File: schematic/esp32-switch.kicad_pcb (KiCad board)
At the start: 2 copper layers, 80 x 100 mm, 27 parts, among them J1 Direction, J11 Bouton 5v, J17 Bouton Batterie, J2 + - home, J3 a b x y, J4 L R ZL ZR, J5 Joy D, J6 Joy G, J7 Moteur vibration, J8 Batterie, Q1 BC547, U1 ESP32-DevKitC

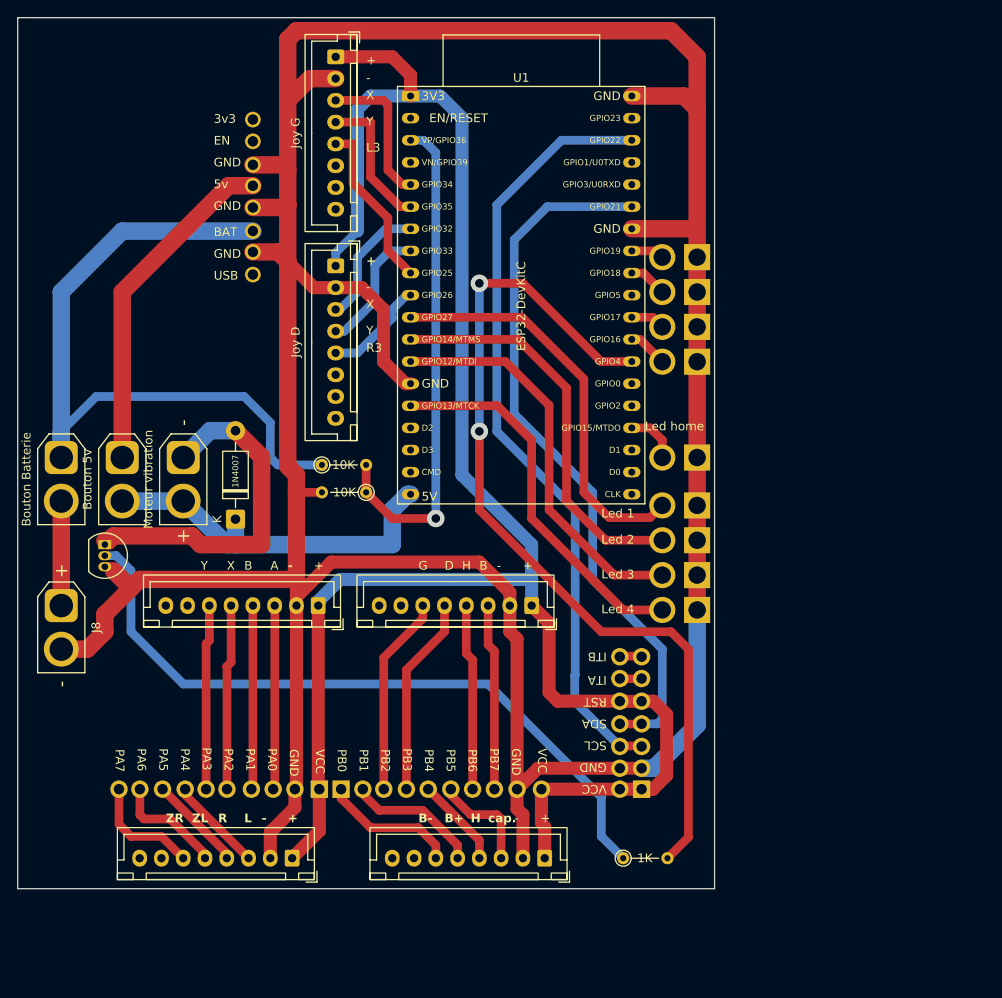
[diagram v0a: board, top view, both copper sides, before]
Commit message: changement de pcb
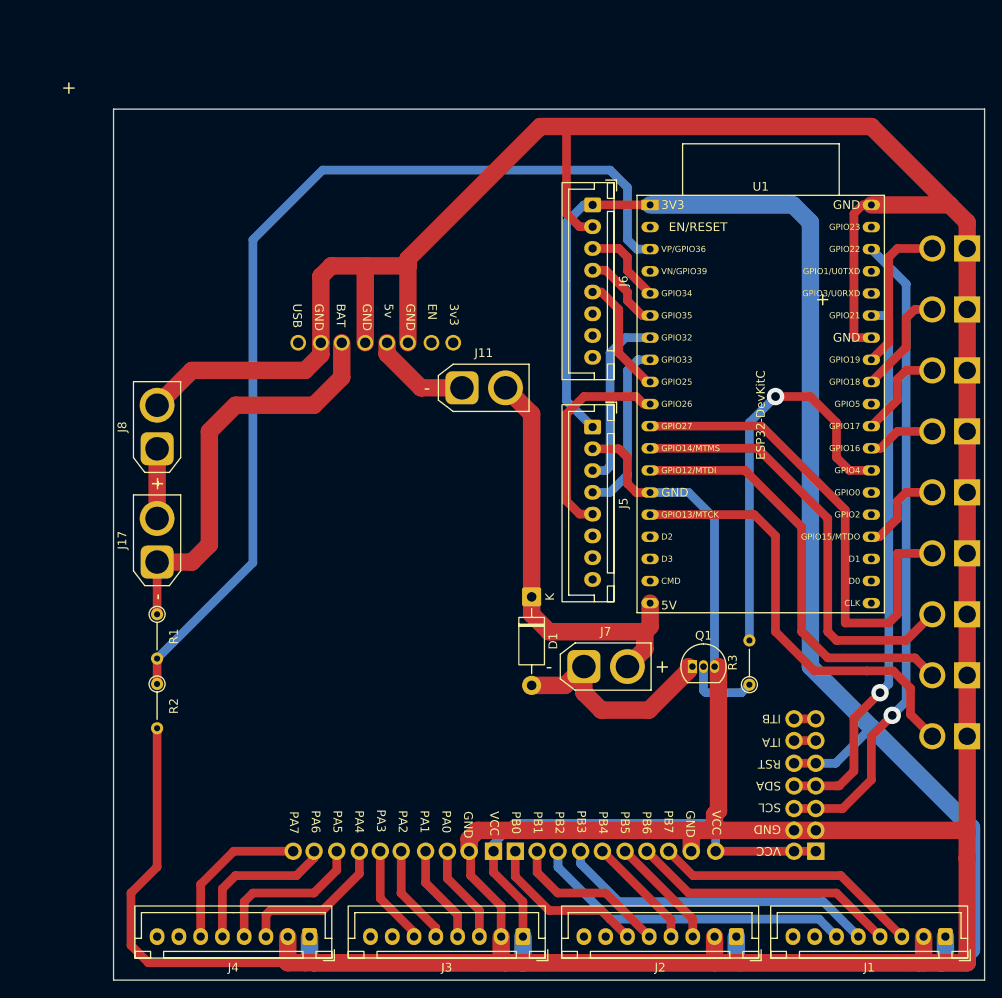
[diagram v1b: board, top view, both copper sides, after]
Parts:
- moved Q1 68.9 mm to (205.5, 105.0), turned to 0 degrees
- moved J1 60.8 mm to (234.5, 136.0)
- moved U2 57.4 mm to (187.0, 43.3), turned to -90 degrees
- moved J7 51.9 mm to (193.0, 105.0), turned to 0 degrees
- moved J3 44.7 mm to (186.0, 136.0)
- moved J11 39.8 mm to (179.0, 73.0), turned to 0 degrees
- moved D1 35.2 mm to (187.0, 97.0), turned to -90 degrees
- moved J5 34.8 mm to (194.0, 77.5)
- moved Led1 34.2 mm to (238.5, 111.5)
- moved J6 34.0 mm to (194.0, 52.0)
- moved Led3 33.1 mm to (238.5, 104.5)
- moved R2 32.6 mm to (144.0, 107.0), turned to -90 degrees
- moved Led2 32.1 mm to (238.5, 97.5)
- moved Led9 32.0 mm to (238.5, 76.5)
- moved Led5 31.5 mm to (238.5, 90.5)
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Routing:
- net Net-(J1-Pin_2): track 387.4 -> 528.0 mm
- net Net-(J1-Pin_1): track 215.5 -> 298.5 mm
- net Net-(Q1-B): track 80.6 -> 8.49 mm
- net Net-(U1-ADC2_CH0/GPIO4): track 102.8 -> 46.1 mm, vias 2 -> 1
- net Net-(U1-SENSOR_VP/GPIO36/ADC1_CH0): track 57.9 -> 111.7 mm, vias 1 -> 0
- net Net-(J17-Pin_1): track 84.1 -> 47.6 mm
- net Net-(J11-Pin_1): track 39.1 -> 11.5 mm
- net Net-(U1-GPIO21): track 82.2 -> 63.4 mm, vias 0 -> 1
- net Net-(D1-A): track 40.2 -> 25.1 mm
- net Net-(U1-GPIO22): track 89.1 -> 74.5 mm, vias 0 -> 1
- net Net-(U1-GPIO19): track 3.80 -> 18.0 mm
- net Net-(J1-Pin_6): track 22.9 -> 37.1 mm
- net Net-(J1-Pin_5): track 22.9 -> 36.8 mm
- net Net-(J5-Pin_5): track 11.5 -> 24.4 mm
- net Net-(U1-ADC2_CH7/GPIO27): track 46.6 -> 56.8 mm
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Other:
- board size 80 x 100 mm -> 100 x 100 mm
- board text removed: "+"
- board text removed: "-"
- board text removed: "A"
- board text removed: "B"
- board text removed: "B+"
- board text removed: "B-"
- board text removed: "D"
- board text removed: "G"
- board text removed: "H"
- board text removed: "L"
- board text removed: "L3"
- board text removed: "Led 1"
- board text removed: "Led 2"
- board text removed: "Led 3"
- board text removed: "Led 4"
- board text removed: "Led home"
- board text removed: "R"
- board text removed: "R3"
- board text removed: "X"
- board text removed: "Y"
- board text removed: "ZL"
- board text removed: "ZR"
- board text removed: "cap."
